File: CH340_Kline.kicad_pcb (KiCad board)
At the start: 2 copper layers, 36.7 x 18.9 mm, 10 parts, among them J1 Conn_01x06, J2 Conn_01x04, Q1 BC847, Q2 BC847

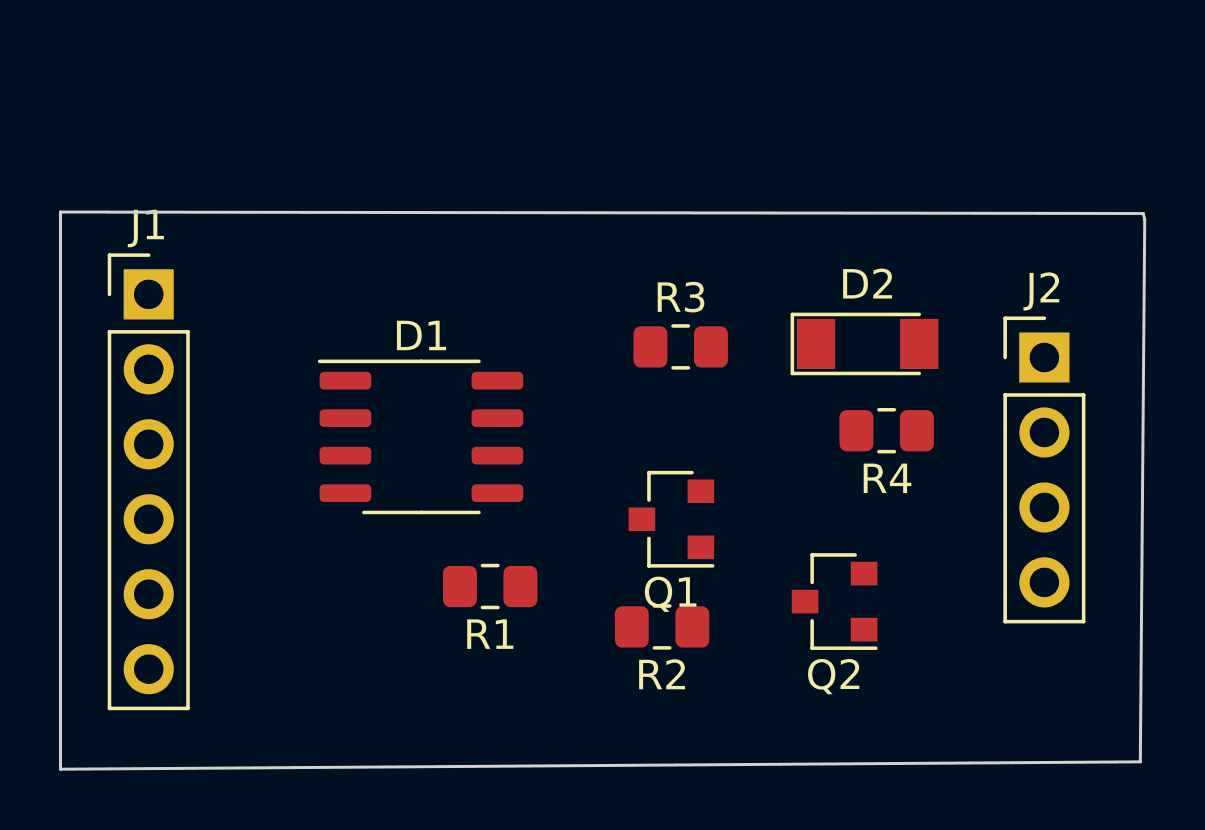
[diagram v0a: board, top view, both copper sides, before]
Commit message: routing complite
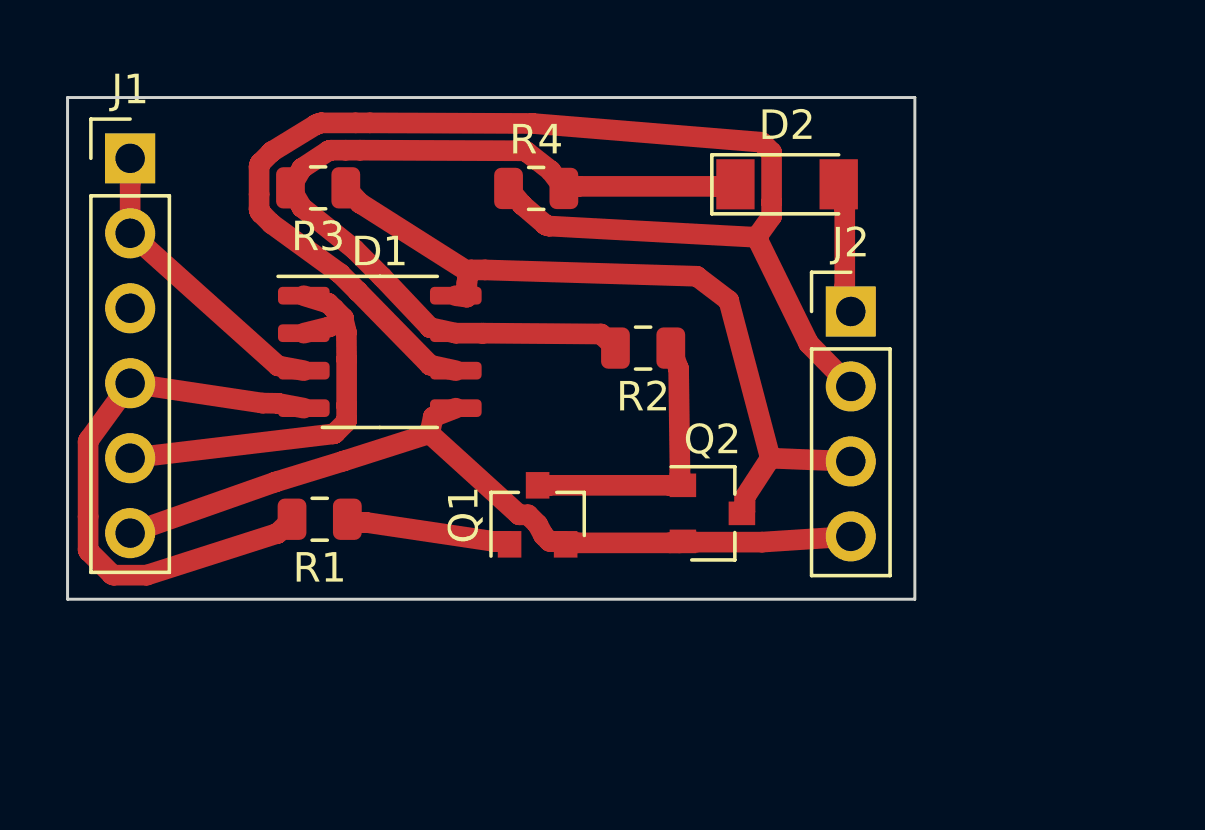
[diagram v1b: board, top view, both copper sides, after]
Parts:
- D1: value L9613 -> L9637D
- R1, R2, R3, R4: footprint Resistor_SMD:R_0805_2012Metric_Pad1.15x1.40mm_HandSolder -> Resistor_SMD:R_0805_2012Metric
- moved R4 14.4 mm to (90.9, 83.1), turned to 0 degrees
- moved R3 13.4 mm to (83.5, 83.1), turned to 180 degrees
- moved R2 9.47 mm to (94.5, 88.5)
- moved J2 6.74 mm to (101.5, 87.2)
- moved R1 6.21 mm to (83.5, 94.3)
- moved D2 6.06 mm to (99.4, 82.9)
- moved Q2 5.11 mm to (96.8, 94.1), turned to 0 degrees
- moved J1 4.65 mm to (77.1, 82.1)
- moved Q1 4.53 mm to (90.9, 94.1), turned to 90 degrees
- moved D1 3.21 mm to (85.6, 88.6)
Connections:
- D1 pad 3: Vcc -> 5V
- J1 pad 1: Rx -> 5V
- J1 pad 2: Tx -> 5V
- J1 pad 3: GND -> 3.3V
- J1 pad 4: 5V -> Tx
- J1 pad 5: Vcc -> Rx
- J1 pad 6: 3.3V -> GND
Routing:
- net K-line: track 0.00 -> 46.3 mm
- net Vss: track 0.00 -> 29.4 mm
- net GND: track 0.00 -> 28.0 mm
- net L-line: track 0.00 -> 25.9 mm
- net Tx: track 0.00 -> 19.7 mm
- net Rx: track 0.00 -> 14.1 mm
- net 5V: track 0.00 -> 10.2 mm
- net Net-(Q1-Pad3): track 0.00 -> 9.68 mm
- net Net-(Q1-Pad1): track 0.00 -> 5.64 mm
- net Net-(D2-Pad2): track 0.00 -> 4.39 mm
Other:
- board size 36.7 x 18.9 mm -> 28.7 x 17 mm
- net class Default: clearance 0.2 -> 0.15; trace_width 0.25 -> 0.7
- rule trace_clearance: 0.2 -> 0.15
